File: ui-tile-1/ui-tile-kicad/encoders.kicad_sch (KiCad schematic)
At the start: 8 parts, among them SW3 EC11E15244G1, SW4 EC11E15244G1, SW5 EC11E15244G1, SW6 EC11E15244G1

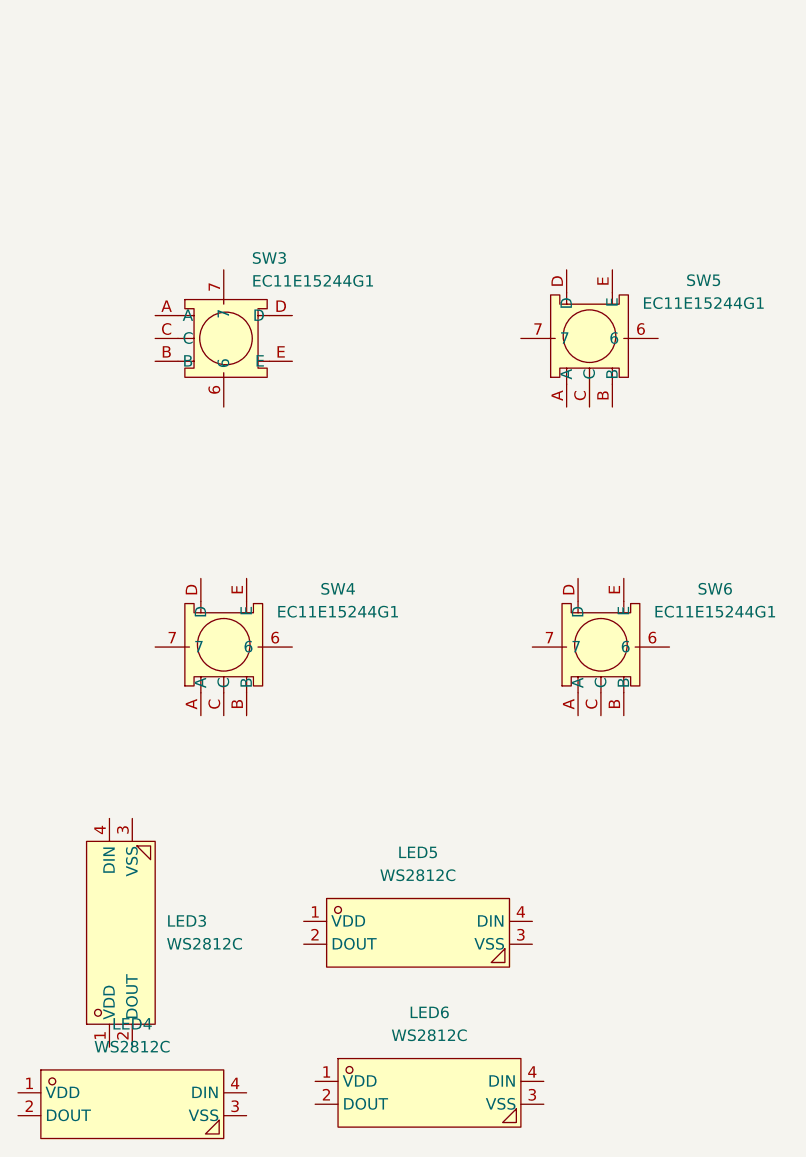
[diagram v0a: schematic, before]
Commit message: finished schematic electricals
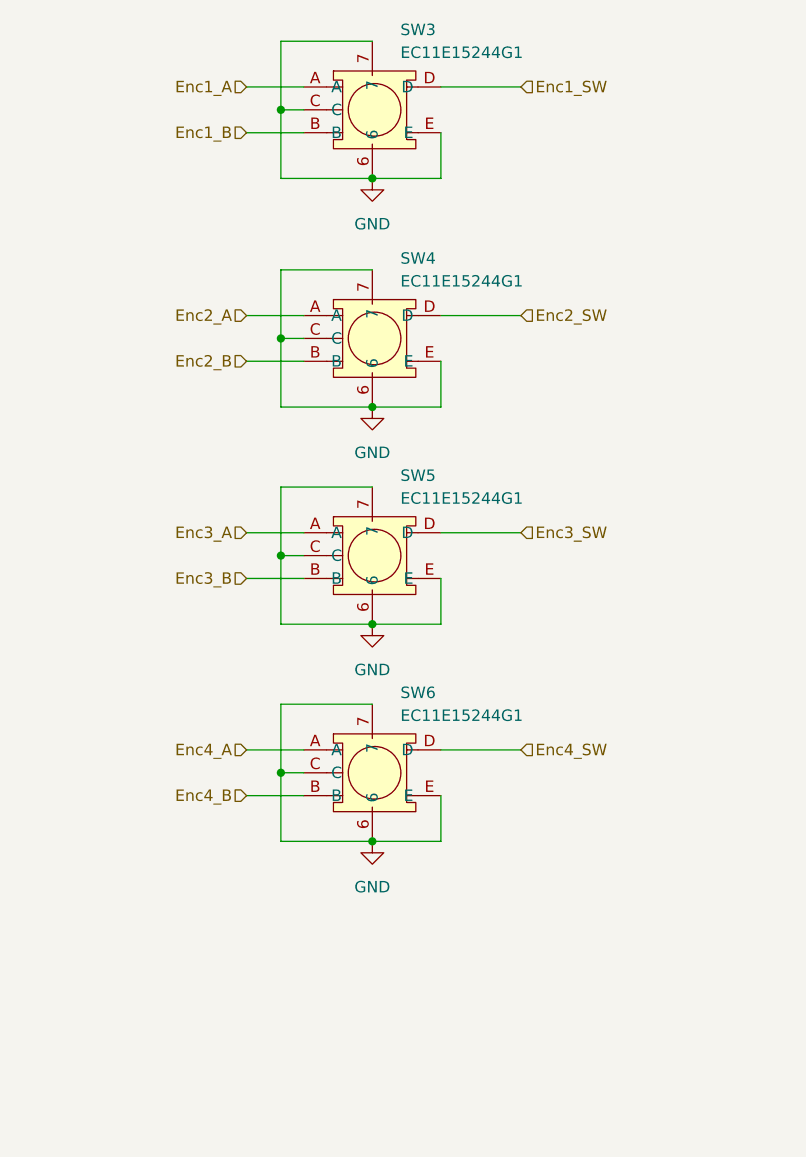
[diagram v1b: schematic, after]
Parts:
- removed LED3, LED4, LED5, LED6: WS2812C, jlcpcb:LED-SMD_4P-L5.0-W5.0-LS5.4-TL-1, symbol jlcpcb:WS2812C
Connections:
- net GND: now reaches SW5.6
- net GND: now also SW3.6, SW3.7, SW3.C, SW3.E, SW4.6, SW4.7, SW4.C, SW4.E, SW5.7, SW5.C, SW5.E, SW6.6, SW6.7, SW6.C, SW6.E
- net Enc3_A: now reaches SW5.A
- net Enc3_B: now reaches SW5.B
- net Enc3_SW: now reaches SW5.D
- net Enc4_A: now reaches SW6.A
- net Enc4_B: now reaches SW6.B
- net Enc4_SW: now reaches SW6.D
- net Enc1_A: now reaches SW3.A
- net Enc1_B: now reaches SW3.B
- net Enc1_SW: now reaches SW3.D
- net Enc2_A: now reaches SW4.A
- net Enc2_B: now reaches SW4.B
- net Enc2_SW: now reaches SW4.D
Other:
- moved on the sheet: SW3
